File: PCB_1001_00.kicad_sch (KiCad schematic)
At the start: 10 parts, among them SW1 SW_MEC_5G, SW2 SW_MEC_5G, SW3 SW_MEC_5G

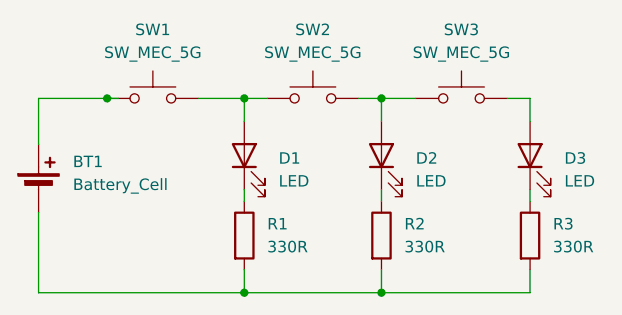
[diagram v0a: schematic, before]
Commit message: PCB_1001_01 routing completed
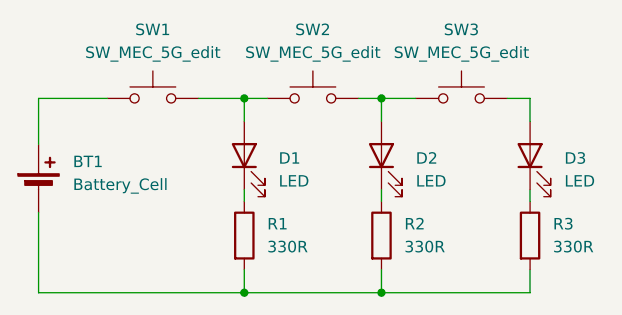
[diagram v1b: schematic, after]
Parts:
- removed SW1, SW2, SW3: SW_MEC_5G, Button_Switch_SMD:SW_Tactile_SPST_NO_Straight_CK_PTS636Sx25SMTRLFS, symbol Switch:SW_MEC_5G
- added SW1, SW2, SW3: SW_MEC_5G_edit, Button_Switch_SMD:SW_Tactile_SPST_NO_Straight_CK_PTS636Sx25SMTRLFS, symbol Sym_Library:SW_MEC_5G_edit
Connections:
- net at D3.2 (A): now also SW3.2 (B)
- net at D1.2 (A): now also SW1.2 (B), SW2.1 (A)
- net at D2.2 (A): now also SW2.2 (B), SW3.1 (A)
- net at BT1.1 (+): now also SW1.1 (A)
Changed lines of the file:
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@@
 	(paper "A4")
-	(junction
-		(at 135.89 88.9)
-		(diameter 0)
-		(color 0 0 0 0)
-	)
 	(junction
 		(at 151.13 110.49)
@@
 	(wire
 		(pts
+			(xy 128.27 88.9) (xy 135.89 88.9)
+		)
+		(stroke
+			(width 0)
+			(type default)
+		)
+	)
+	(wire
+		(pts
 			(xy 163.83 88.9) (xy 166.37 88.9)
 		)
@@
 	(wire
 		(pts
-			(xy 137.16 88.9) (xy 135.89 88.9)
-		)
-		(stroke
-			(width 0)
-			(type default)
-		)
-	)
-	(wire
-		(pts
 			(xy 128.27 88.9) (xy 128.27 93.98)
 		)
@@
 	(wire
 		(pts
-			(xy 135.89 88.9) (xy 128.27 88.9)
-		)
-		(stroke
-			(width 0)
-			(type default)
-		)
-	)
-	(wire
-		(pts
 			(xy 182.88 88.9) (xy 182.88 91.44)
 		)
@@
 			(width 0)
 			(type default)
+		)
+	)
+	(symbol
+		(lib_id "Sym_Library:SW_MEC_5G_edit")
+		(at 175.26 88.9 0)
+		(unit 1)
+		(exclude_from_sim no)
+		(in_bom yes)
+		(on_board yes)
+		(dnp no)
+		(fields_autoplaced yes)
+		(property "Reference" "SW3"
+			(at 175.26 81.28 0)
+			(effects
+				(font
+					(size 1.27 1.27)
+				)
+			)
+		)
+		(property "Value" "SW_MEC_5G_edit"
+			(at 175.26 83.82 0)
+			(effects
+				(font
+					(size 1.27 1.27)
+				)
+			)
+		)
+		(property "Footprint" "Button_Switch_SMD:SW_Tactile_SPST_NO_Straight_CK_PTS636Sx25SMTRLFS"
+			(at 175.26 83.82 0)
+			(effects
+				(font
+					(size 1.27 1.27)
+				)
+				(hide yes)
+			)
+		)
+		(property "Datasheet" "http://www.apem.com/int/index.php?controller=attachment&id_attachment=488"
+			(at 175.26 83.82 0)
+			(effects
+				(font
+					(size 1.27 1.27)
+				)
+				(hide yes)
+			)
+		)
+		(property "Description" "MEC 5G single pole normally-open tactile switch"
+			(at 175.26 88.9 0)
+			(effects
+				(font
+					(size 1.27 1.27)
+				)
+				(hide yes)
+			)
+		)
+		(pin "1"
+		)
+		(pin "2"
+		)
+		(instances
+			(project ""
+				(path "/9c4608c9-b9d4-4f6a-9cb6-835175086c03"
+					(reference "SW3")
+					(unit 1)
+				)
+			)
+		)
+	)
+	(symbol
+		(lib_id "Sym_Library:SW_MEC_5G_edit")
+		(at 140.97 88.9 0)
+		(unit 1)
+		(exclude_from_sim no)
+		(in_bom yes)
+		(on_board yes)
+		(dnp no)
+		(fields_autoplaced yes)
+		(property "Reference" "SW1"
+			(at 140.97 81.28 0)
+			(effects
+				(font
+					(size 1.27 1.27)
+				)
+			)
+		)
+		(property "Value" "SW_MEC_5G_edit"
+			(at 140.97 83.82 0)
+			(effects
+				(font
+					(size 1.27 1.27)
+				)
+			)
+		)
+		(property "Footprint" "Button_Switch_SMD:SW_Tactile_SPST_NO_Straight_CK_PTS636Sx25SMTRLFS"
+			(at 140.97 83.82 0)
+			(effects
+				(font
+					(size 1.27 1.27)
+				)
+				(hide yes)
+			)
+		)
+		(property "Datasheet" "http://www.apem.com/int/index.php?controller=attachment&id_attachment=488"
+			(at 140.97 83.82 0)
+			(effects
+				(font
+					(size 1.27 1.27)
+				)
+				(hide yes)
+			)
+		)
+		(property "Description" "MEC 5G single pole normally-open tactile switch"
+			(at 140.97 88.9 0)
+			(effects
+				(font
+					(size 1.27 1.27)
+				)
+				(hide yes)
+			)
+		)
+		(pin "2"
+		)
+		(pin "1"
+		)
+		(instances
+			(project ""
+				(path "/9c4608c9-b9d4-4f6a-9cb6-835175086c03"
+					(reference "SW1")
+					(unit 1)
+				)
+			)
 		)
 	)
@@
 	)
 	(symbol
-		(lib_id "Switch:SW_MEC_5G")
+		(lib_id "Sym_Library:SW_MEC_5G_edit")
 		(at 158.75 88.9 0)
 		(unit 1)
@@
 			)
 		)
-		(property "Value" "SW_MEC_5G"
+		(property "Value" "SW_MEC_5G_edit"
 			(at 158.75 83.82 0)
 			(effects
@@
 			)
 		)
-		(pin "3"
-		)
-		(pin "2"
-		)
-		(pin "1"
-		)
-		(pin "4"
-		)
-		(instances
-			(project "PCB_1001_00"
+		(pin "1"
+		)
+		(pin "2"
+		)
+		(instances
+			(project ""
 				(path "/9c4608c9-b9d4-4f6a-9cb6-835175086c03"
 					(reference "SW2")
-					(unit 1)
-				)
-			)
-		)
-	)
-	(symbol
-		(lib_id "Switch:SW_MEC_5G")
-		(at 140.97 88.9 0)
-		(unit 1)
-		(exclude_from_sim no)
-		(in_bom yes)
-		(on_board yes)
-		(dnp no)
-		(fields_autoplaced yes)
-		(property "Reference" "SW1"
-			(at 140.97 81.28 0)
-			(effects
-				(font
-					(size 1.27 1.27)
-				)
-			)
-		)
-		(property "Value" "SW_MEC_5G"
-			(at 140.97 83.82 0)
-			(effects
-				(font
-					(size 1.27 1.27)
-				)
-			)
-		)
-		(property "Footprint" "Button_Switch_SMD:SW_Tactile_SPST_NO_Straight_CK_PTS636Sx25SMTRLFS"
-			(at 140.97 83.82 0)
-			(effects
-				(font
-					(size 1.27 1.27)
-				)
-				(hide yes)
-			)
-		)
-		(property "Datasheet" "http://www.apem.com/int/index.php?controller=attachment&id_attachment=488"
-			(at 140.97 83.82 0)
-			(effects
-				(font
-					(size 1.27 1.27)
-				)
-				(hide yes)
-			)
-		)
-		(property "Description" "MEC 5G single pole normally-open tactile switch"
-			(at 140.97 88.9 0)
-			(effects
-				(font
-					(size 1.27 1.27)
-				)
-				(hide yes)
-			)
-		)
-		(pin "3"
-		)
-		(pin "2"
-		)
-		(pin "1"
-		)
-		(pin "4"
-		)
-		(instances
-			(project ""
-				(path "/9c4608c9-b9d4-4f6a-9cb6-835175086c03"
-					(reference "SW1")
 					(unit 1)
 				)
@@
 					(unit 1)
 				)
-			)
-		)
-	)
-	(symbol
-		(lib_id "Switch:SW_MEC_5G")
-		(at 175.26 88.9 0)
-		(unit 1)
-		(exclude_from_sim no)
-		(in_bom yes)
-		(on_board yes)
-		(dnp no)
-		(fields_autoplaced yes)
-		(property "Reference" "SW3"
-			(at 175.26 81.28 0)
-			(effects
-				(font
-					(size 1.27 1.27)
-				)
-			)
-		)
-		(property "Value" "SW_MEC_5G"
-			(at 175.26 83.82 0)
-			(effects
-				(font
-					(size 1.27 1.27)
-				)
-			)
-		)
-		(property "Footprint" "Button_Switch_SMD:SW_Tactile_SPST_NO_Straight_CK_PTS636Sx25SMTRLFS"
-			(at 175.26 83.82 0)
-			(effects
-				(font
-					(size 1.27 1.27)
-				)
-				(hide yes)
-			)
-		)
-		(property "Datasheet" "http://www.apem.com/int/index.php?controller=attachment&id_attachment=488"
-			(at 175.26 83.82 0)
-			(effects
-				(font
-					(size 1.27 1.27)
-				)
-				(hide yes)
-			)
-		)
-		(property "Description" "MEC 5G single pole normally-open tactile switch"
-			(at 175.26 88.9 0)
-			(effects
-				(font
-					(size 1.27 1.27)
-				)
-				(hide yes)
-			)
-		)
-		(pin "3"
-		)
-		(pin "2"
-		)
-		(pin "1"
-		)
-		(pin "4"
-		)
-		(instances
-			(project "PCB_1001_00"
-				(path "/9c4608c9-b9d4-4f6a-9cb6-835175086c03"
-					(reference "SW3")
-					(unit 1)
-				)
